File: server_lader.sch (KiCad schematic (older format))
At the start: 27 parts

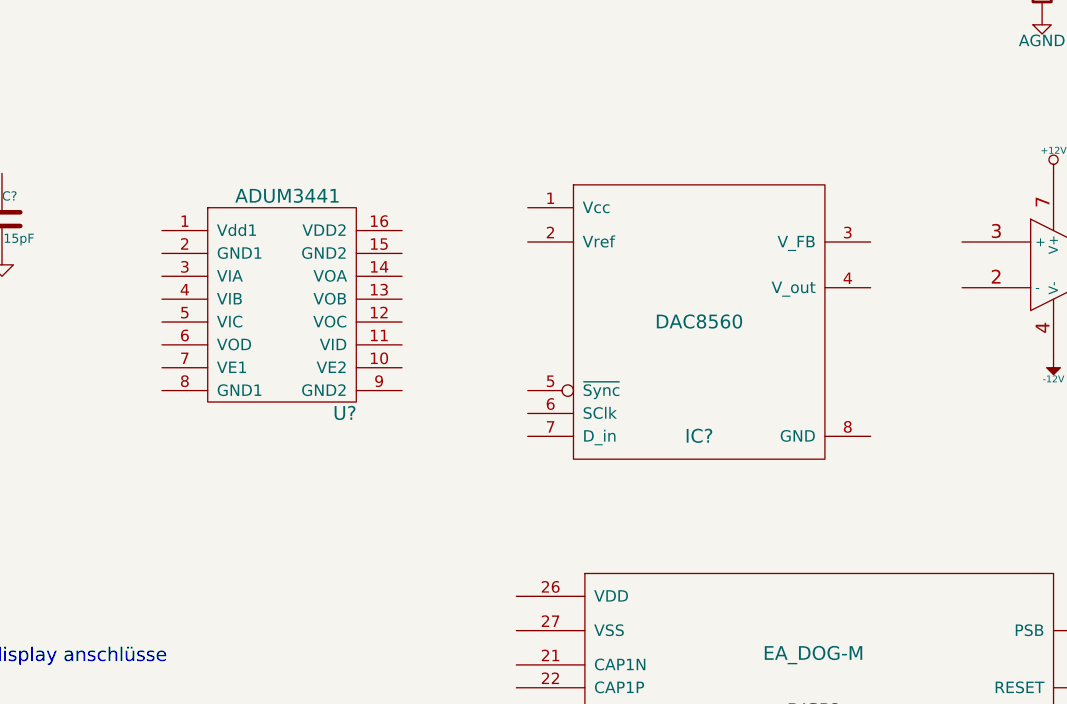
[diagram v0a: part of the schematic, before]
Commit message: work
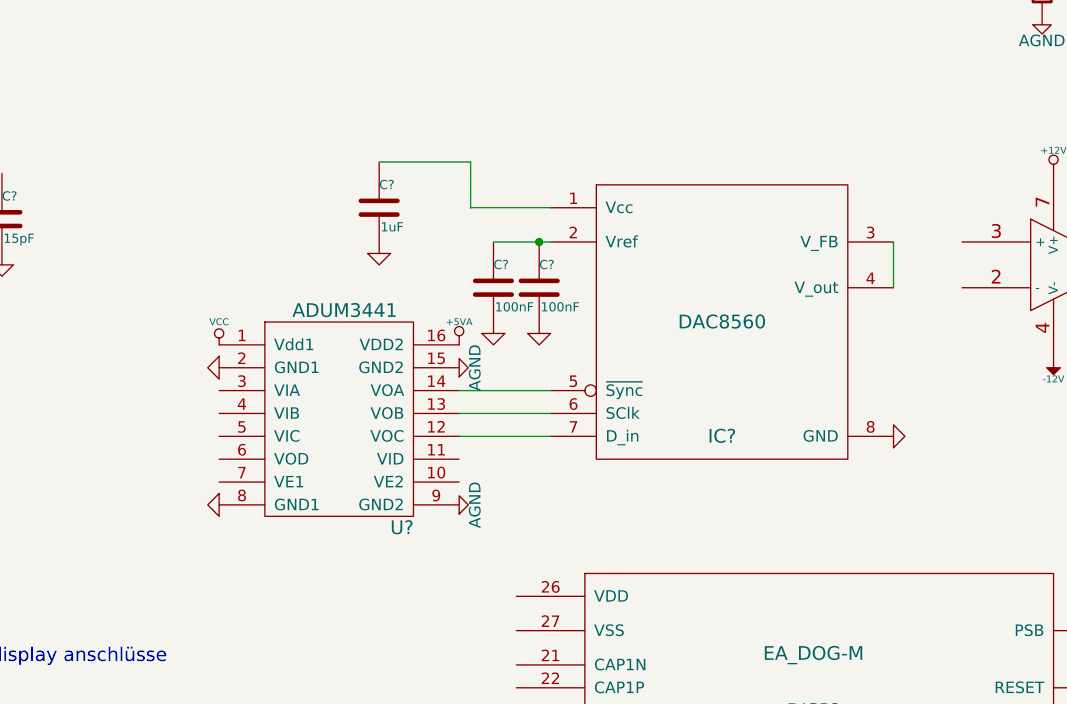
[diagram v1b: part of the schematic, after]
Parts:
- added C?: 1uF, symbol C
- added C? (x2): 100nF, symbol C
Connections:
- wire segments 42 -> 50
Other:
- moved on the sheet: IC?, U?
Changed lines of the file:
@@
 L DAC8560 IC?
 U 1 1 5462BFB9
-P 8950 3400
-F 0 "IC?" H 8950 2900 60  0000 C CNN
-F 1 "DAC8560" H 8950 3400 60  0000 C CNN
-F 2 "" H 7700 2650 60  0000 C CNN
-F 3 "" H 7700 2650 60  0000 C CNN
-	1    8950 3400
+P 9050 3400
+F 0 "IC?" H 9050 2900 60  0000 C CNN
+F 1 "DAC8560" H 9050 3400 60  0000 C CNN
+F 2 "" H 7800 2650 60  0000 C CNN
+F 3 "" H 7800 2650 60  0000 C CNN
+	1    9050 3400
 	1    0    0    -1
 $EndComp
@@
 L ADUM3441 U?
 U 1 1 5462CAA6
-P 7100 3200
-F 0 "U?" H 7400 2600 60  0000 C CNN
-F 1 "ADUM3441" H 7150 3550 60  0000 C CNN
-F 2 "" H 6850 3200 60  0000 C CNN
-F 3 "" H 6850 3200 60  0000 C CNN
-	1    7100 3200
+P 7350 3700
+F 0 "U?" H 7650 3100 60  0000 C CNN
+F 1 "ADUM3441" H 7400 4050 60  0000 C CNN
+F 2 "" H 7100 3700 60  0000 C CNN
+F 3 "" H 7100 3700 60  0000 C CNN
+	1    7350 3700
 	1    0    0    -1
 $EndComp
@@
 	1    0    0    -1
 $EndComp
+Wire Wire Line
+	7900 3700 8300 3700
+Wire Wire Line
+	7900 3800 8300 3800
+Wire Wire Line
+	7900 3900 8300 3900
+$Comp
+L AGND #PWR?
+U 1 1 5462B7A5
+P 7900 4200
+F 0 "#PWR?" H 7900 4200 40  0001 C CNN
+F 1 "AGND" H 7900 4130 50  0000 C CNN
+F 2 "" H 7900 4200 60  0000 C CNN
+F 3 "" H 7900 4200 60  0000 C CNN
+	1    7900 4200
+	0    -1   -1   0
+$EndComp
+$Comp
+L AGND #PWR?
+U 1 1 5462B837
+P 7900 3600
+F 0 "#PWR?" H 7900 3600 40  0001 C CNN
+F 1 "AGND" H 7900 3530 50  0000 C CNN
+F 2 "" H 7900 3600 60  0000 C CNN
+F 3 "" H 7900 3600 60  0000 C CNN
+	1    7900 3600
+	0    -1   -1   0
+$EndComp
+$Comp
+L +5VA #PWR?
+U 1 1 5462B9BC
+P 7900 3500
+F 0 "#PWR?" H 7900 3630 20  0001 C CNN
+F 1 "+5VA" H 7900 3600 30  0000 C CNN
+F 2 "" H 7900 3500 60  0000 C CNN
+F 3 "" H 7900 3500 60  0000 C CNN
+	1    7900 3500
+	1    0    0    -1
+$EndComp
+$Comp
+L VCC #PWR?
+U 1 1 5462BAA9
+P 6850 3500
+F 0 "#PWR?" H 6850 3600 30  0001 C CNN
+F 1 "VCC" H 6850 3600 30  0000 C CNN
+F 2 "" H 6850 3500 60  0000 C CNN
+F 3 "" H 6850 3500 60  0000 C CNN
+	1    6850 3500
+	1    0    0    -1
+$EndComp
+$Comp
+L GND #PWR?
+U 1 1 5462BB3B
+P 6850 3600
+F 0 "#PWR?" H 6850 3600 30  0001 C CNN
+F 1 "GND" H 6850 3530 30  0001 C CNN
+F 2 "" H 6850 3600 60  0000 C CNN
+F 3 "" H 6850 3600 60  0000 C CNN
+	1    6850 3600
+	0    1    1    0
+$EndComp
+$Comp
+L GND #PWR?
+U 1 1 5462BB61
+P 6850 4200
+F 0 "#PWR?" H 6850 4200 30  0001 C CNN
+F 1 "GND" H 6850 4130 30  0001 C CNN
+F 2 "" H 6850 4200 60  0000 C CNN
+F 3 "" H 6850 4200 60  0000 C CNN
+	1    6850 4200
+	0    1    1    0
+$EndComp
+$Comp
+L C C?
+U 1 1 5462C075
+P 7550 2900
+F 0 "C?" H 7550 3000 40  0000 L CNN
+F 1 "1uF" H 7556 2815 40  0000 L CNN
+F 2 "" H 7588 2750 30  0000 C CNN
+F 3 "" H 7550 2900 60  0000 C CNN
+	1    7550 2900
+	1    0    0    -1
+$EndComp
+$Comp
+L C C?
+U 1 1 5462C2DF
+P 8250 3250
+F 0 "C?" H 8250 3350 40  0000 L CNN
+F 1 "100nF" H 8256 3165 40  0000 L CNN
+F 2 "" H 8288 3100 30  0000 C CNN
+F 3 "" H 8250 3250 60  0000 C CNN
+	1    8250 3250
+	1    0    0    -1
+$EndComp
+$Comp
+L C C?
+U 1 1 5462C429
+P 8050 3250
+F 0 "C?" H 8050 3350 40  0000 L CNN
+F 1 "100nF" H 8056 3165 40  0000 L CNN
+F 2 "" H 8088 3100 30  0000 C CNN
+F 3 "" H 8050 3250 60  0000 C CNN
+	1    8050 3250
+	1    0    0    -1
+$EndComp
+Wire Wire Line
+	8050 3050 8300 3050
+$Comp
+L GND #PWR?
+U 1 1 5462C4B3
+P 8250 3450
+F 0 "#PWR?" H 8250 3450 30  0001 C CNN
+F 1 "GND" H 8250 3380 30  0001 C CNN
+F 2 "" H 8250 3450 60  0000 C CNN
+F 3 "" H 8250 3450 60  0000 C CNN
+	1    8250 3450
+	1    0    0    -1
+$EndComp
+$Comp
+L GND #PWR?
+U 1 1 5462C4DC
+P 8050 3450
+F 0 "#PWR?" H 8050 3450 30  0001 C CNN
+F 1 "GND" H 8050 3380 30  0001 C CNN
+F 2 "" H 8050 3450 60  0000 C CNN
+F 3 "" H 8050 3450 60  0000 C CNN
+	1    8050 3450
+	1    0    0    -1
+$EndComp
+$Comp
+L GND #PWR?
+U 1 1 5462C505
+P 7550 3100
+F 0 "#PWR?" H 7550 3100 30  0001 C CNN
+F 1 "GND" H 7550 3030 30  0001 C CNN
+F 2 "" H 7550 3100 60  0000 C CNN
+F 3 "" H 7550 3100 60  0000 C CNN
+	1    7550 3100
+	1    0    0    -1
+$EndComp
+Wire Wire Line
+	7550 2700 7950 2700
+Wire Wire Line
+	7950 2700 7950 2900
+Wire Wire Line
+	7950 2900 8300 2900
+Connection ~ 8250 3050
+$Comp
+L GND #PWR?
+U 1 1 5462C873
+P 9800 3900
+F 0 "#PWR?" H 9800 3900 30  0001 C CNN
+F 1 "GND" H 9800 3830 30  0001 C CNN
+F 2 "" H 9800 3900 60  0000 C CNN
+F 3 "" H 9800 3900 60  0000 C CNN
+	1    9800 3900
+	0    -1   -1   0
+$EndComp
+Wire Wire Line
+	9800 3250 9800 3050
 $EndSCHEMATC
